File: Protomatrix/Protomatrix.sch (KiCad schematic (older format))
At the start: 141 parts, among them J1 Conn_01x21_Female

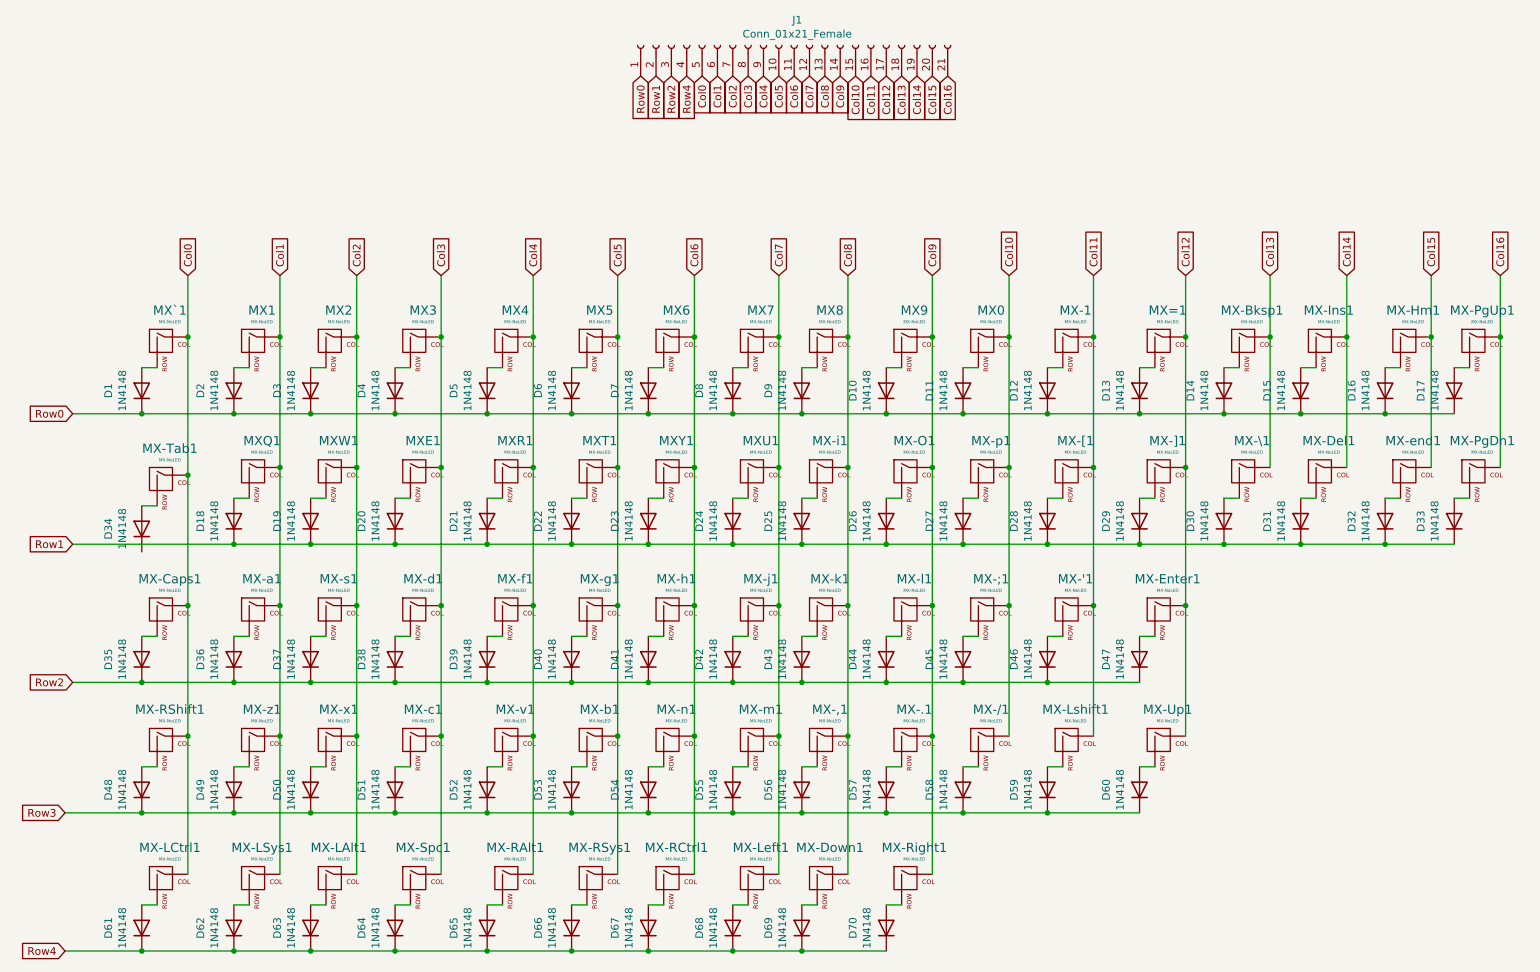
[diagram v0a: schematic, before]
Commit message: Routing and stuff
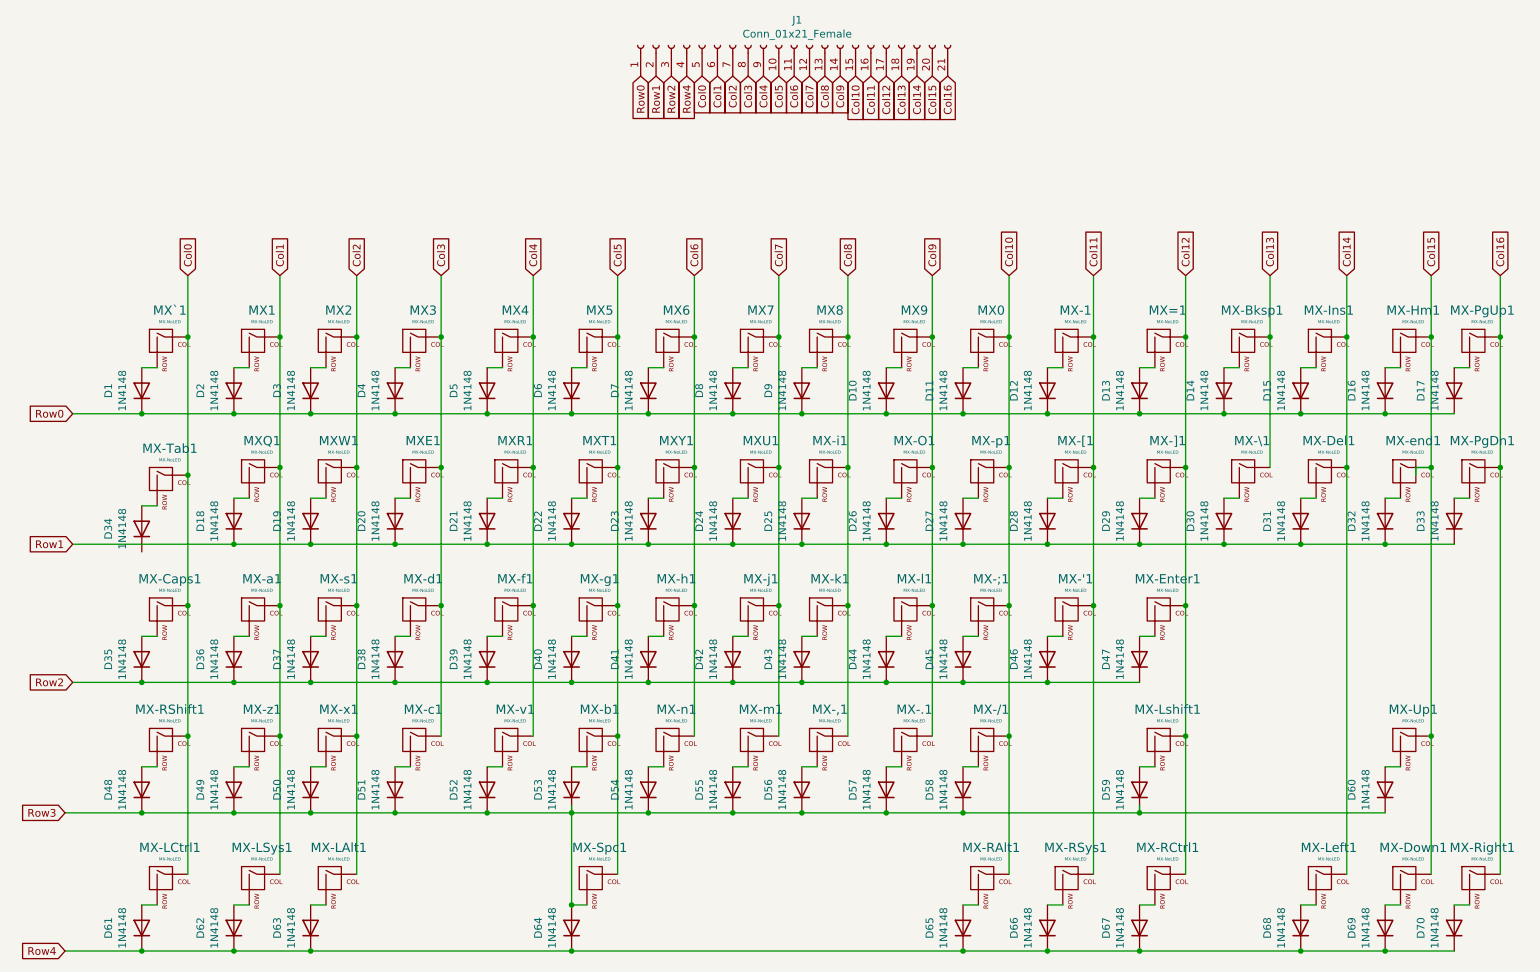
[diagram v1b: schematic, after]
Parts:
- MX-'1, MX-,1, MX-.1, MX-/1, MX-1, MX-;1, MX-Del1, MX-Down1, MX-Hm1, MX-Ins1, MX-LSys1, MX-Left1, MX-O1, MX-PgDn1, MX-PgUp1, MX-RSys1, MX-Right1, MX-Up1, MX-[1, MX-]1, MX-a1, MX-b1, MX-c1, MX-d1, MX-end1, MX-f1, MX-g1, MX-h1, MX-i1, MX-j1, MX-k1, MX-l1, MX-m1, MX-n1, MX-p1, MX-s1, MX-v1, MX-x1, MX-z1, MX0, MX1, MX2, MX3, MX4, MX5, MX6, MX7, MX8, MX9, MX=1, MXE1, MXQ1, MXR1, MXT1, MXU1, MXW1, MXY1, MX`1: footprint (none) -> MX_Only:MXOnly-1U-NoLED
- MX-Bksp1: footprint (none) -> MX_Only:MXOnly-2U-NoLED
- MX-Caps1: footprint (none) -> MX_Only:MXOnly-1.75U-NoLED
- MX-Enter1, MX-Lshift1: footprint (none) -> MX_Only:MXOnly-2.25U-NoLED
- MX-LAlt1, MX-LCtrl1, MX-RAlt1, MX-RCtrl1, MX-Tab1, MX-\1: footprint (none) -> MX_Only:MXOnly-1.5U-NoLED
- MX-RShift1: footprint (none) -> MX_Only:MXOnly-2.75U-NoLED
- MX-Spc1: footprint (none) -> MX_Only:MXOnly-7U-ReversedStabilizers-NoLED
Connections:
- net Col10: now also MX-RAlt1.1 (COL)
- net Col11: now also MX-RSys1.1 (COL); no longer MX-Lshift1.1 (COL)
- net Col12: now also MX-Lshift1.1 (COL), MX-RCtrl1.1 (COL); no longer MX-Up1.1 (COL)
- net Col14: now also MX-Left1.1 (COL)
- net Col15: now also MX-Down1.1 (COL), MX-Up1.1 (COL)
- net Col16: now also MX-Right1.1 (COL)
- net Col3: no longer MX-Spc1.1 (COL)
- net Col4: no longer MX-RAlt1.1 (COL)
- net Col5: now also MX-Spc1.1 (COL); no longer MX-RSys1.1 (COL)
- net Col6: no longer MX-RCtrl1.1 (COL)
- net Col7: no longer MX-Left1.1 (COL)
- net Col8: no longer MX-Down1.1 (COL)
- net Col9: no longer MX-Right1.1 (COL)
- net Row3: now also D64.2 (A), MX-Spc1.2 (ROW)
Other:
- moved on the sheet: D59, D60, D64, D65, D66, D67, D68, D69, D70, MX-Down1, MX-Left1, MX-Lshift1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
